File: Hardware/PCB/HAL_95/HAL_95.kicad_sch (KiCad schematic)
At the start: 0 parts

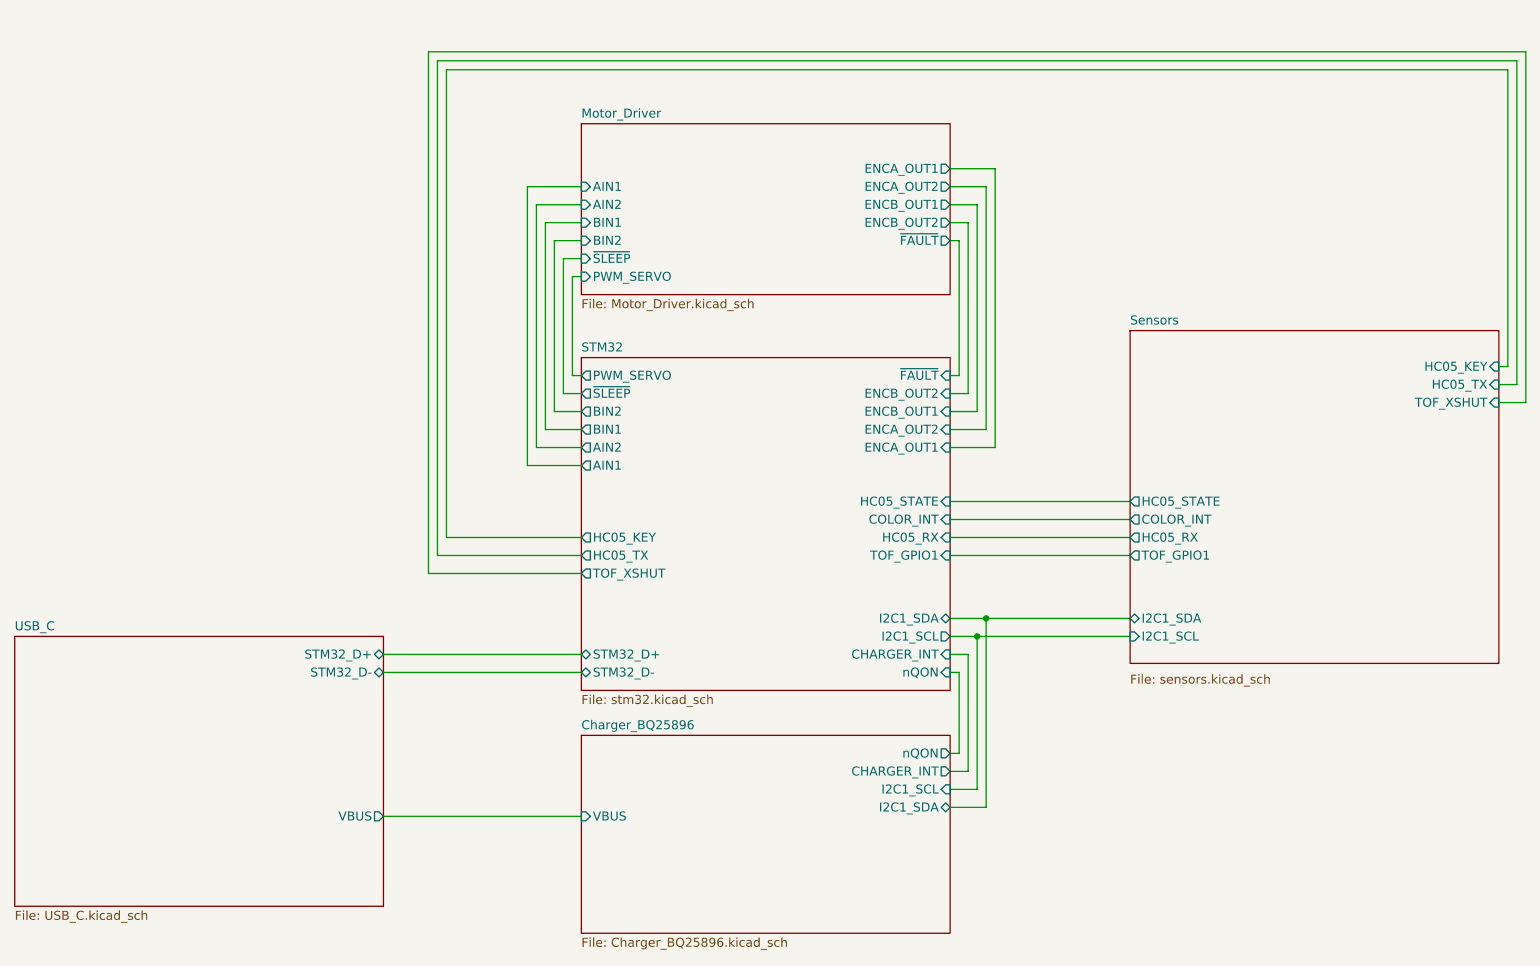
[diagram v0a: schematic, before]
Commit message: finished schematic
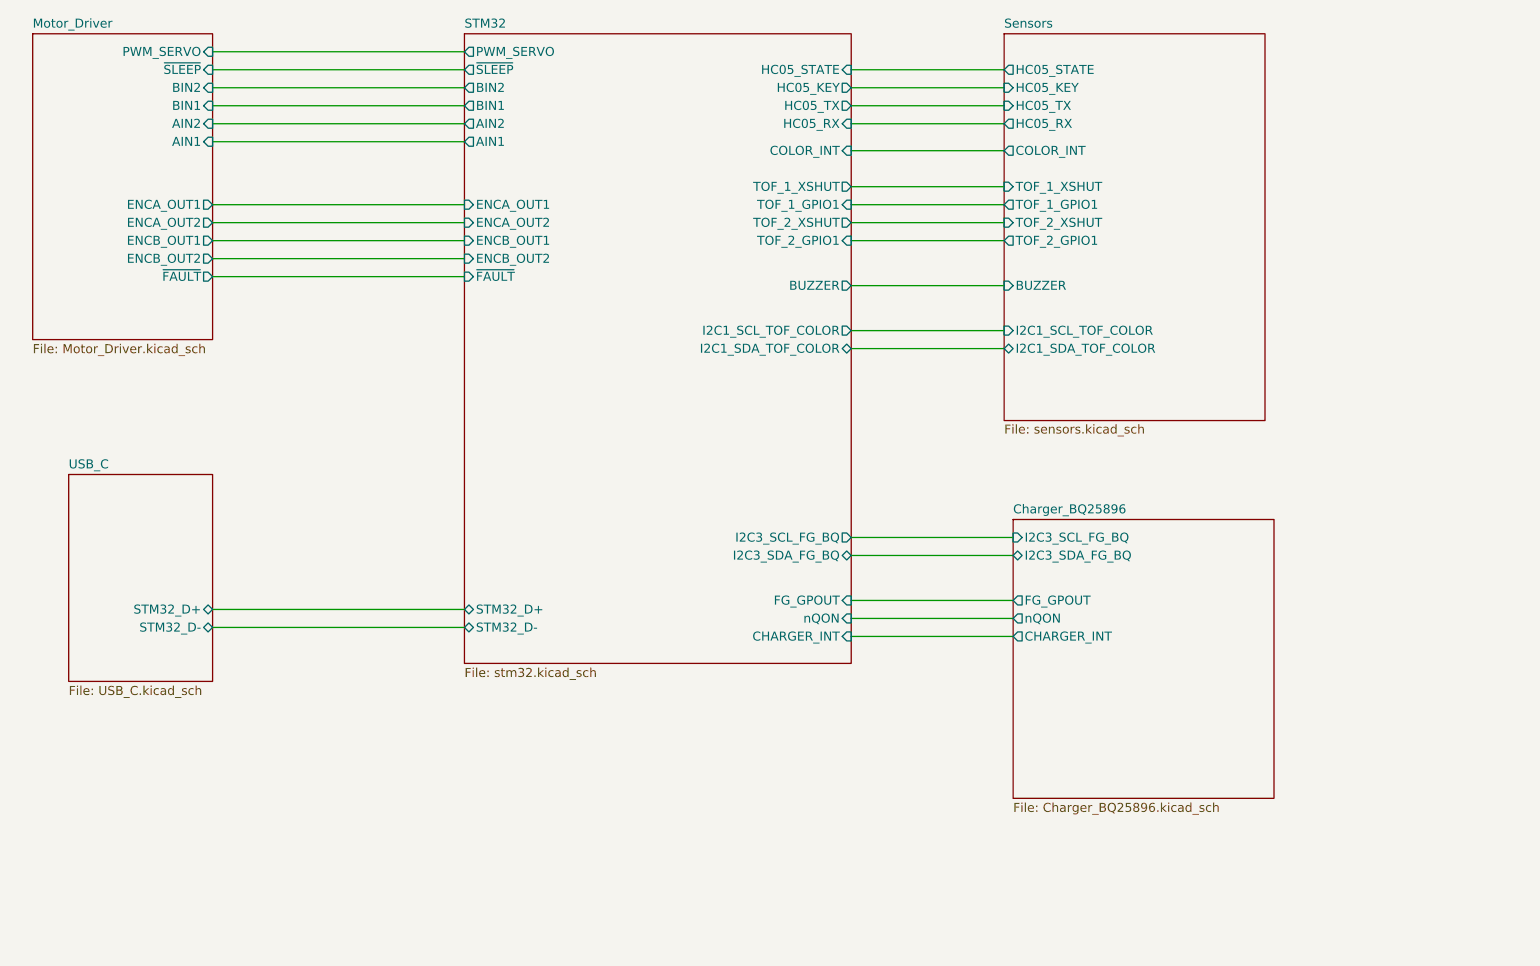
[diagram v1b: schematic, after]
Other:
- sheet Charger_BQ25896 ports: added FG_GPOUT, I2C3_SCL_FG_BQ, I2C3_SDA_FG_BQ; removed I2C1_SCL, I2C1_SDA, VBUS
- sheet STM32 ports: added BUZZER, FG_GPOUT, I2C1_SCL_TOF_COLOR, I2C1_SDA_TOF_COLOR, I2C3_SCL_FG_BQ, I2C3_SDA_FG_BQ, TOF_1_GPIO1, TOF_1_XSHUT, TOF_2_GPIO1, TOF_2_XSHUT; removed I2C1_SCL, I2C1_SDA, TOF_GPIO1, TOF_XSHUT
- sheet Sensors ports: added BUZZER, I2C1_SCL_TOF_COLOR, I2C1_SDA_TOF_COLOR, TOF_1_GPIO1, TOF_1_XSHUT, TOF_2_GPIO1, TOF_2_XSHUT; removed I2C1_SCL, I2C1_SDA, TOF_GPIO1, TOF_XSHUT
- sheet USB_C ports: added none; removed VBUS
